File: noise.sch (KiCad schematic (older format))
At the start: 31 parts, among them U1 4584, U2 TL072, U3 78L05

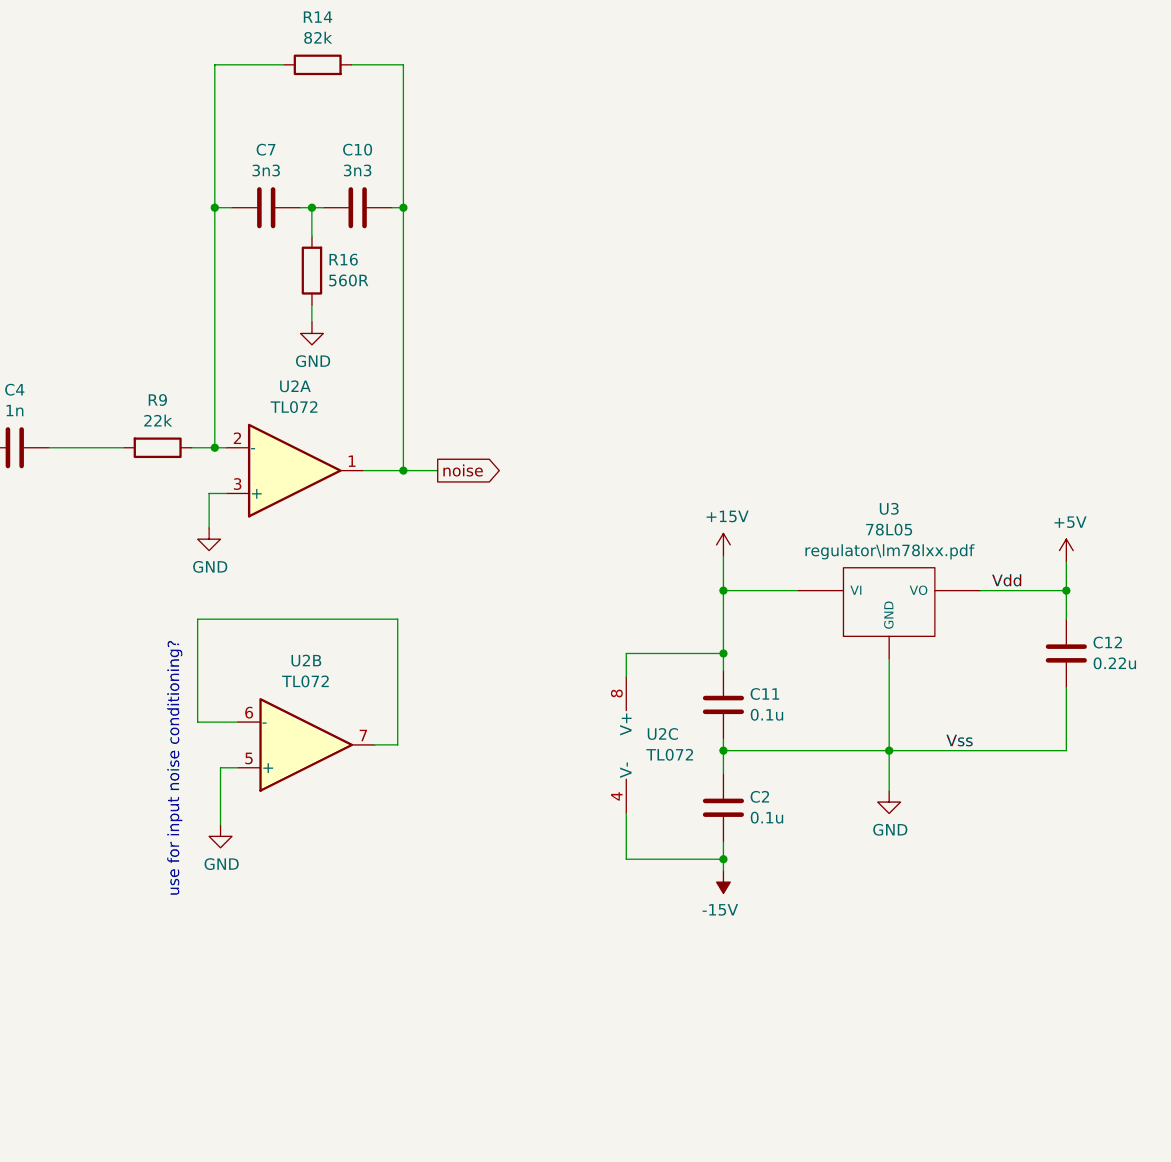
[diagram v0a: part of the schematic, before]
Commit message: noise in/out with selection
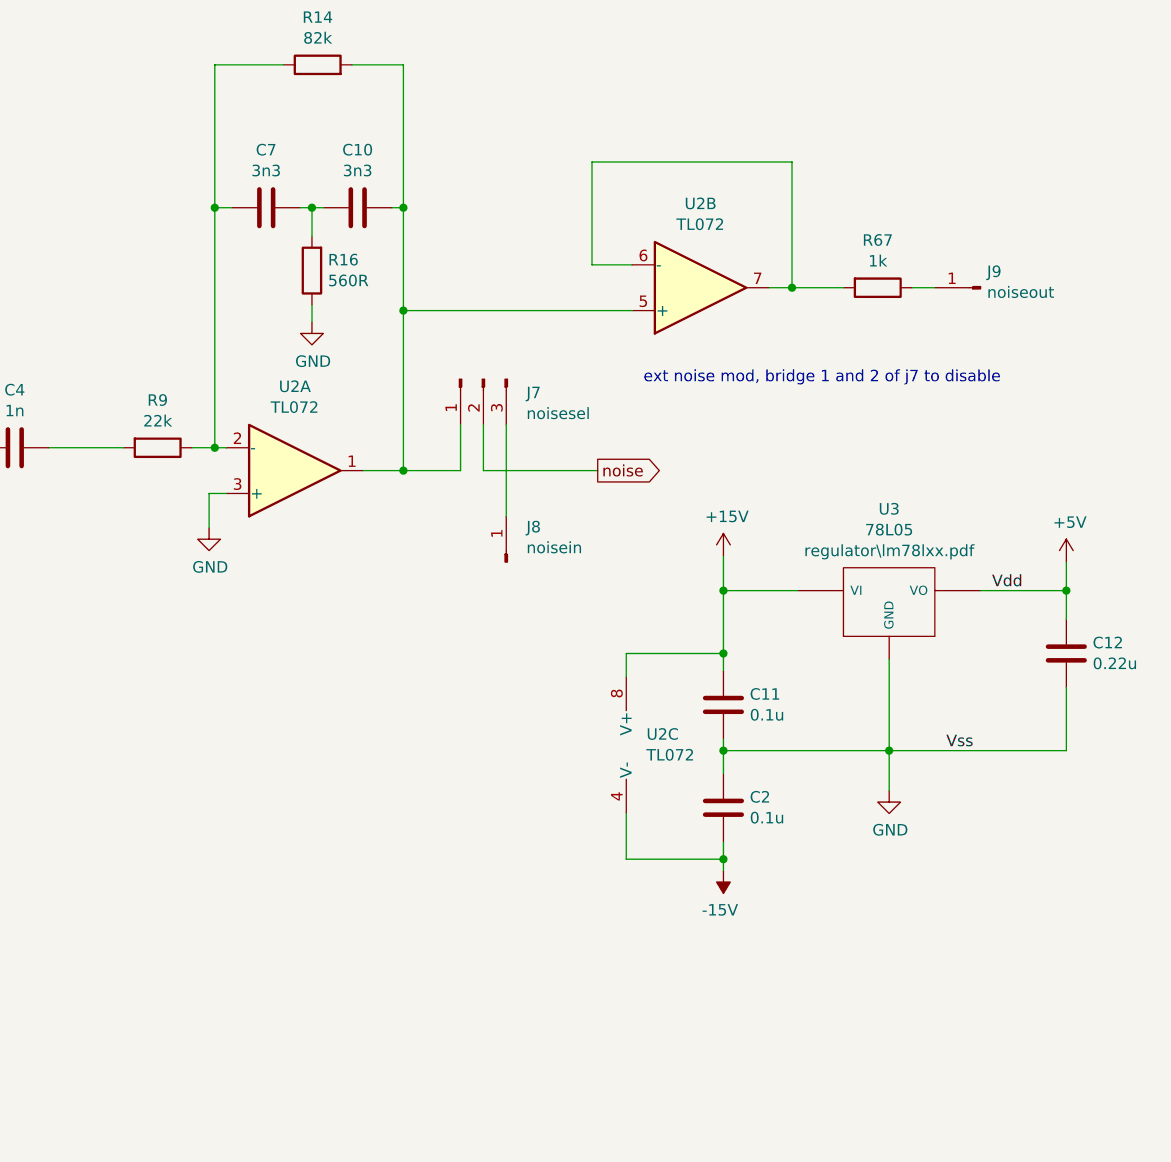
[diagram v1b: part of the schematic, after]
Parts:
- added J7: noisesel, symbol Connector:Conn_01x03_Male
- added J8: noisein, symbol Connector:Conn_01x01_Male
- added J9: noiseout, symbol Connector:Conn_01x01_Male
- added R67: 1k, symbol Device:R
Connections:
- net GND: no longer U2.5 (+)
- net noise: now also J7.2 (Pin_2); no longer C10.1, R14.2, U2.1
- net at U2.6 (-), U2.7: now also R67.2
- new net: J9.1 (Pin_1), R67.1
- new net: C10.1, J7.1 (Pin_1), R14.2, U2.1, U2.5 (+)
- new net: J7.3 (Pin_3), J8.1 (Pin_1)
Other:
- note added: "ext noise mod, bridge 1 and 2 of j7 to disable"
- note removed: "use for input noise conditioning?"
- moved on the sheet: U2B
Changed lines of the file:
@@
 Wire Wire Line
 	4100 3300 3775 3300
-Text GLabel 5475 3400 2    50   Output ~ 0
+Text GLabel 6175 3400 2    50   Output ~ 0
 noise
-Wire Wire Line
-	5475 3400 5325 3400
 $Comp
 L Device:C C7
@@
 	4500 3300 4400 3300
 Wire Wire Line
-	5325 2250 5325 3400
+	5325 2250 5325 2700
 Connection ~ 5325 2250
-Connection ~ 5325 3400
 Wire Wire Line
 	5325 3400 5150 3400
@@
 L Amplifier_Operational:TL072 U2
 U 2 1 5CC85CA2
-P 4900 4600
-F 0 "U2" H 4900 4233 50  0000 C CNN
-F 1 "TL072" H 4900 4324 50  0000 C CNN
-F 2 "" H 4900 4600 50  0001 C CNN
-F 3 "http://www.ti.com/lit/ds/symlink/tl071.pdf" H 4900 4600 50  0001 C CNN
-	2    4900 4600
+P 6625 2600
+F 0 "U2" H 6625 2233 50  0000 C CNN
+F 1 "TL072" H 6625 2324 50  0000 C CNN
+F 2 "" H 6625 2600 50  0001 C CNN
+F 3 "http://www.ti.com/lit/ds/symlink/tl071.pdf" H 6625 2600 50  0001 C CNN
+	2    6625 2600
 	1    0    0    1
 $EndComp
 Wire Wire Line
-	4600 4500 4425 4500
-Wire Wire Line
-	4425 4050 5300 4050
-Wire Wire Line
-	5300 4050 5300 4600
-Wire Wire Line
-	5300 4600 5200 4600
-$Comp
-L power:GND #PWR0146
-U 1 1 5CC886A6
-P 4525 4950
-F 0 "#PWR0146" H 4525 4700 50  0001 C CNN
-F 1 "GND" H 4530 4777 50  0000 C CNN
-F 2 "" H 4525 4950 50  0001 C CNN
-F 3 "" H 4525 4950 50  0001 C CNN
-	1    4525 4950
-	1    0    0    -1
-$EndComp
-Wire Wire Line
-	4600 4700 4525 4700
-Wire Wire Line
-	4525 4700 4525 4950
+	6325 2500 6150 2500
+Wire Wire Line
+	6150 2050 7025 2050
+Wire Wire Line
+	7025 2050 7025 2600
+Wire Wire Line
+	7025 2600 6925 2600
 $Comp
 L Amplifier_Operational:TL072 U2
@@
 Connection ~ 2950 2350
 Wire Wire Line
-	4425 4500 4425 4050
-Text Notes 4350 4150 3    50   ~ 0
-use for input noise conditioning?
+	6150 2500 6150 2050
+Wire Wire Line
+	5325 2700 6325 2700
+Connection ~ 5325 2700
+Wire Wire Line
+	5325 2700 5325 3400
+$Comp
+L Device:R R67
+U 1 1 5CB9F9E2
+P 7400 2600
+F 0 "R67" V 7193 2600 50  0000 C CNN
+F 1 "1k" V 7284 2600 50  0000 C CNN
+F 2 "" V 7330 2600 50  0001 C CNN
+F 3 "~" H 7400 2600 50  0001 C CNN
+	1    7400 2600
+	0    1    1    0
+$EndComp
+Wire Wire Line
+	7250 2600 7025 2600
+Connection ~ 7025 2600
+$Comp
+L Connector:Conn_01x01_Male J9
+U 1 1 5CBA38EB
+P 7850 2600
+F 0 "J9" H 7822 2530 50  0000 R CNN
+F 1 "noiseout" H 7822 2621 50  0000 R CNN
+F 2 "" H 7850 2600 50  0001 C CNN
+F 3 "~" H 7850 2600 50  0001 C CNN
+	1    7850 2600
+	-1   0    0    1
+$EndComp
+Wire Wire Line
+	7550 2600 7650 2600
+$Comp
+L Connector:Conn_01x03_Male J7
+U 1 1 5CBAF9DC
+P 5675 3000
+F 0 "J7" V 5735 2812 50  0000 R CNN
+F 1 "noisesel" V 5826 2812 50  0000 R CNN
+F 2 "" H 5675 3000 50  0001 C CNN
+F 3 "~" H 5675 3000 50  0001 C CNN
+	1    5675 3000
+	0    -1   1    0
+$EndComp
+Wire Wire Line
+	5575 3200 5575 3400
+Wire Wire Line
+	5575 3400 5325 3400
+Connection ~ 5325 3400
+Wire Wire Line
+	5675 3200 5675 3400
+Wire Wire Line
+	5675 3400 6175 3400
+$Comp
+L Connector:Conn_01x01_Male J8
+U 1 1 5CBBB5C9
+P 5775 3800
+F 0 "J8" V 5928 3712 50  0000 R CNN
+F 1 "noisein" V 5837 3712 50  0000 R CNN
+F 2 "" H 5775 3800 50  0001 C CNN
+F 3 "~" H 5775 3800 50  0001 C CNN
+	1    5775 3800
+	0    -1   -1   0
+$EndComp
+Wire Wire Line
+	5775 3200 5775 3600
+Text Notes 6375 3025 0    50   ~ 0
+ext noise mod, bridge 1 and 2 of j7 to disable
 $EndSCHEMATC
